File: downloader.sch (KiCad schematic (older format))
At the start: 16 parts, among them J1 USB_C_Receptacle_USB2.0, J2 Conn_01x06_Female, Q1 SS8050-G, Q2 SS8050-G, SW1 SW_Push, SW2 SW_Push, U1 AMS1117-3.3, U2 ch340k

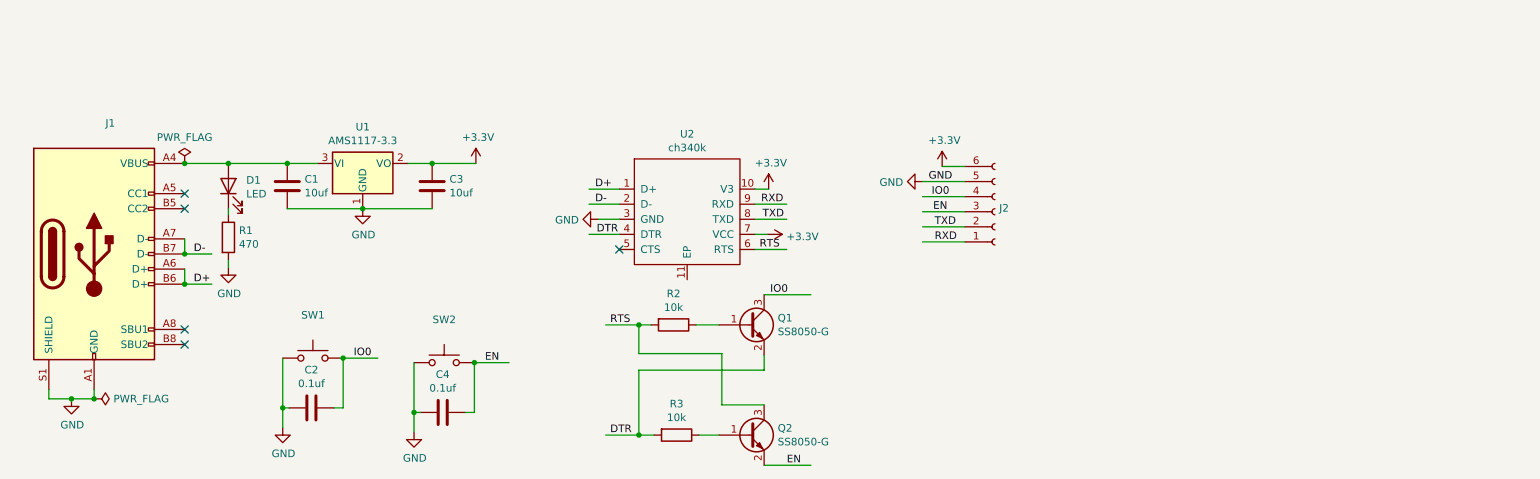
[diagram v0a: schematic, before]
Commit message: version2.0
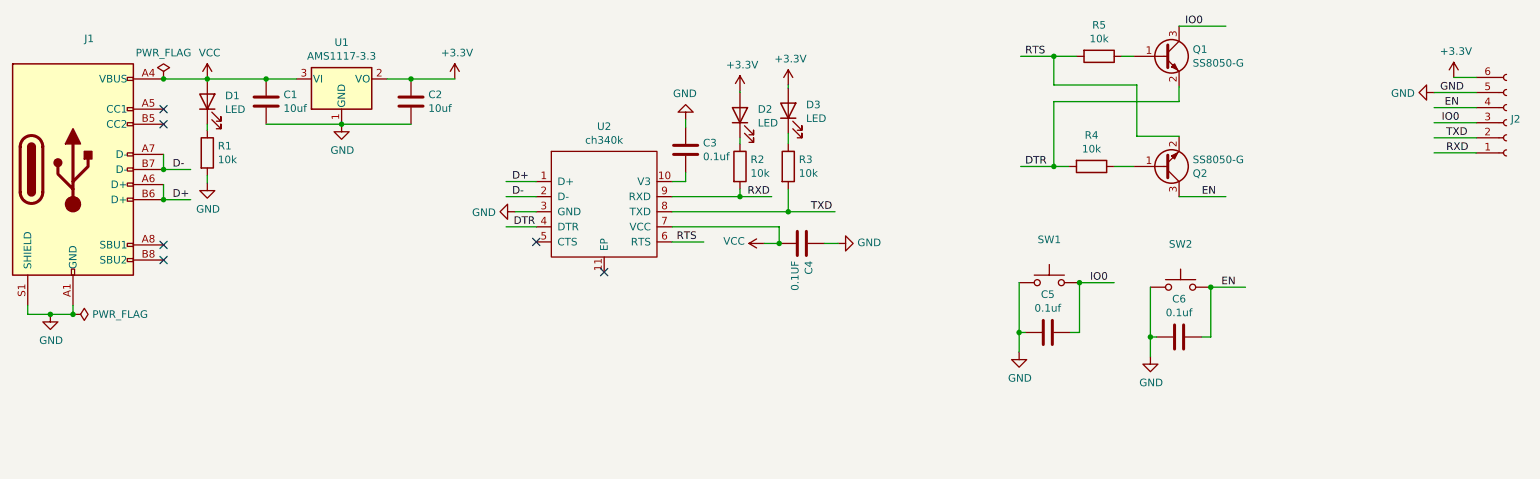
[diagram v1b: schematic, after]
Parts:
- added C3: 0.1uf, Capacitor_SMD:C_0603_1608Metric, symbol Device:C
- added C4: 0.1UF, Capacitor_SMD:C_0603_1608Metric, symbol Device:C
- added D2, D3: LED, Diode_SMD:D_0603_1608Metric, symbol Device:LED
- added R3, R5: 10k, Resistor_SMD:R_0603_1608Metric, symbol Device:R
- R1: value 470 -> 10k
- U2: footprint Package_SO:SSOP-10_3.9x4.9mm_P1.00mm -> my:ESSOP-10_3.9x4.9mm_P1.00mm
- renumbered C3 to C2, C2 to C5, C4 to C6, R3 to R4
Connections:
- net labels added: VCC
- wire segments 59 -> 72
- no-connect marks 5 -> 6
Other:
- moved on the sheet: C1, C2, C5, C6, D1, J1, J2, Q1, Q2, R1, R4, SW1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
